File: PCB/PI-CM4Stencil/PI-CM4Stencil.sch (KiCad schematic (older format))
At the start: 2 parts

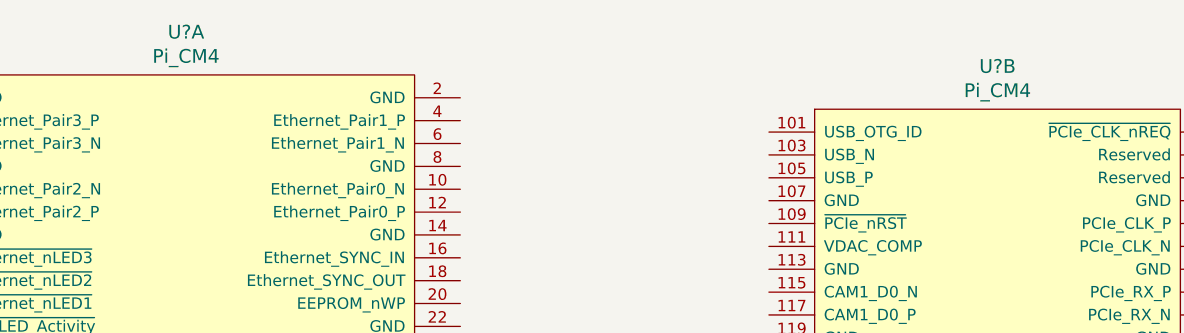
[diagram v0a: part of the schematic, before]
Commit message: Created gerber files
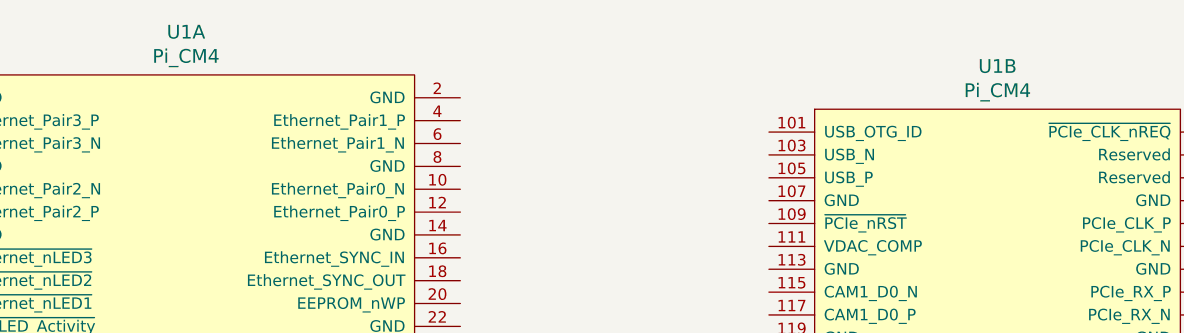
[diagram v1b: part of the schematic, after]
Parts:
- U1: renamed from U?; footprint (none) -> PI-CM4Stencil:Pi_CM4
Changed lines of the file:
@@
 $EndDescr
 $Comp
-L PI-CM4Stencil:Pi_CM4 U?
+L PI-CM4Stencil:Pi_CM4 U1
 U 1 1 61E11F1A
 P 2650 1150
-F 0 "U?" H 3850 1437 60  0000 C CNN
+F 0 "U1" H 3850 1437 60  0000 C CNN
 F 1 "Pi_CM4" H 3850 1331 60  0000 C CNN
-F 2 "" H 2850 1200 60  0001 L CNN
+F 2 "PI-CM4Stencil:Pi_CM4" H 2850 1200 60  0001 L CNN
 F 3 "" H 2850 1000 60  0001 L CNN
 	1    2650 1150
@@
 $EndComp
 $Comp
-L PI-CM4Stencil:Pi_CM4 U?
+L PI-CM4Stencil:Pi_CM4 U1
 U 2 1 61E1AEBE
 P 6400 1300
-F 0 "U?" H 7400 1587 60  0000 C CNN
+F 0 "U1" H 7400 1587 60  0000 C CNN
 F 1 "Pi_CM4" H 7400 1481 60  0000 C CNN
-F 2 "" H 6600 1350 60  0001 L CNN
+F 2 "PI-CM4Stencil:Pi_CM4" H 6600 1350 60  0001 L CNN
 F 3 "" H 6600 1150 60  0001 L CNN
 	2    6400 1300
